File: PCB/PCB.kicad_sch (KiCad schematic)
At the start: 45 parts, among them J1 Conn_01x04_Pin, J2 Conn_01x01, J3 Conn_01x08, J4 Conn_01x02, J6 Conn_01x04, SW1 PTS815SJM250SMTRLFS, SW2 PTS815SJM250SMTRLFS, U1 IQS7222A001QNR, U6 AP63203WU, U7 ESP32-C3-WROOM-02

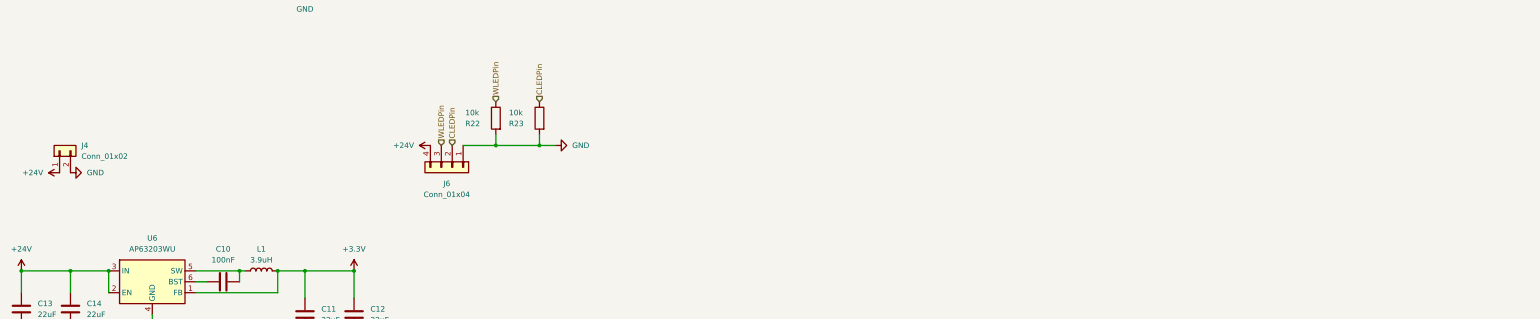
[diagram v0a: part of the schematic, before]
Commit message: commit
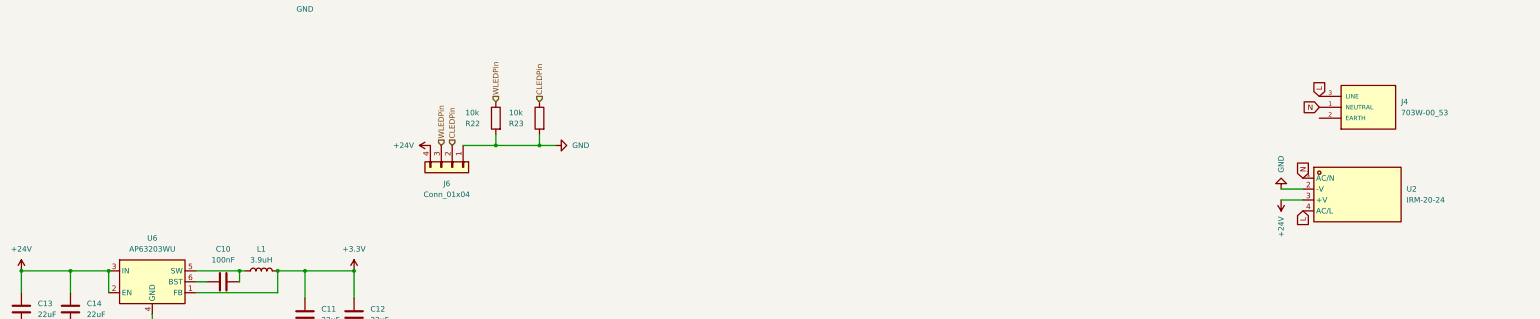
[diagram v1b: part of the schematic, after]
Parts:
- removed J4: Conn_01x02, Connector_JST:JST_XH_B2B-XH-AM_1x02_P2.50mm_Vertical, symbol Connector_Generic:Conn_01x02
- added J4: 703W-00_53, Extra:QUALTEK_703W-00_53, symbol Extra:703W-00_53
- added U2: IRM-20-24, easyeda2kicad:PWRM-TH_IRM-20-24, symbol easyeda2kicad:IRM-20-24
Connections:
- net +24V: now also U2.3 (+V)
- net GND: now also U2.2 (-V)
- new net L: J4.3 (LINE), U2.4 (AC/L)
- new net N: J4.1 (NEUTRAL), U2.1 (AC/N)
